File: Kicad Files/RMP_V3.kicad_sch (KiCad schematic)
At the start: 16 parts, among them U2 ATMega2560

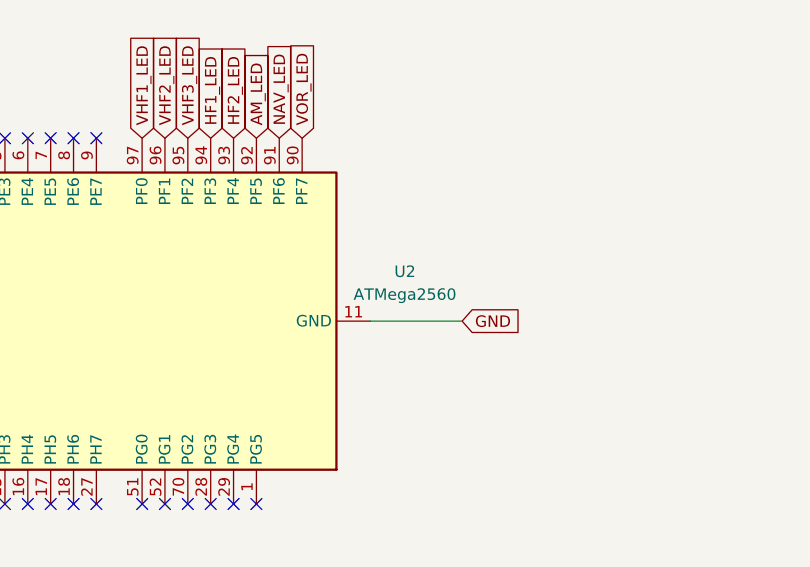
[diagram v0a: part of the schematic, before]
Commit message: Various updates and fixes
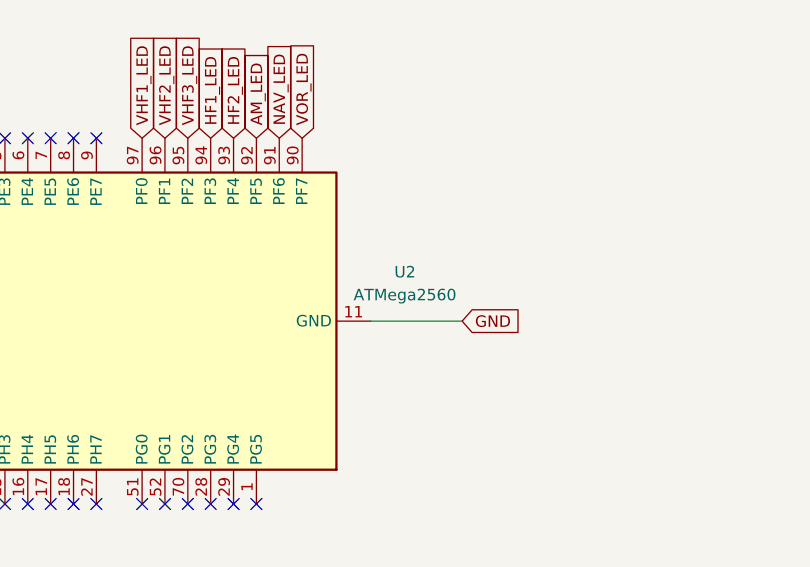
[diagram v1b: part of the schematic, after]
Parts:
- U2: footprint SFLibrary:TQFP100-0.5-14X14MM -> Package_QFP:TQFP-100_14x14mm_P0.5mm
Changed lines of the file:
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@@
 (kicad_sch
-	(version 20231120)
+	(version 20250114)
 	(generator "eeschema")
-	(generator_version "8.0")
+	(generator_version "9.0")
 	(paper "A4")
 	(junction
@@
 		(fields_autoplaced yes)
 		(property "Reference" "U2"
-			(at 231.14 91.0238 90)
+			(at 231.14 91.0746 90)
 			(effects
 				(font
@@
 		)
 		(property "Value" "ATMega2560"
-			(at 231.14 93.5638 90)
+			(at 231.14 93.6146 90)
 			(effects
 				(font
@@
 			)
 		)
-		(property "Footprint" "SFLibrary:TQFP100-0.5-14X14MM"
+		(property "Footprint" "Package_QFP:TQFP-100_14x14mm_P0.5mm"
 			(at 153.67 96.52 0)
 			(effects
@@
 		(at -1.27 226.06)
 		(size 298.45 193.04)
+		(exclude_from_sim no)
+		(in_bom yes)
+		(on_board yes)
+		(dnp no)
 		(fields_autoplaced yes)
 		(stroke
@@
 		(at 598.17 229.87)
 		(size 260.35 187.96)
+		(exclude_from_sim no)
+		(in_bom yes)
+		(on_board yes)
+		(dnp no)
 		(fields_autoplaced yes)
 		(stroke
@@
 		(at 303.53 0)
 		(size 280.67 208.28)
+		(exclude_from_sim no)
+		(in_bom yes)
+		(on_board yes)
+		(dnp no)
 		(fields_autoplaced yes)
 		(stroke
@@
 		(at 596.9 0)
 		(size 261.62 207.01)
+		(exclude_from_sim no)
+		(in_bom yes)
+		(on_board yes)
+		(dnp no)
 		(fields_autoplaced yes)
 		(stroke
@@
 		)
 	)
+	(embedded_fonts no)
 )
